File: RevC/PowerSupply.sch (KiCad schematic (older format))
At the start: 26 parts, among them Q21 DMG2301L, U22 TPS54202, U23 L7805, U24 MCP1754ST-3302E/CB, U25 NCP51460SN33T1G

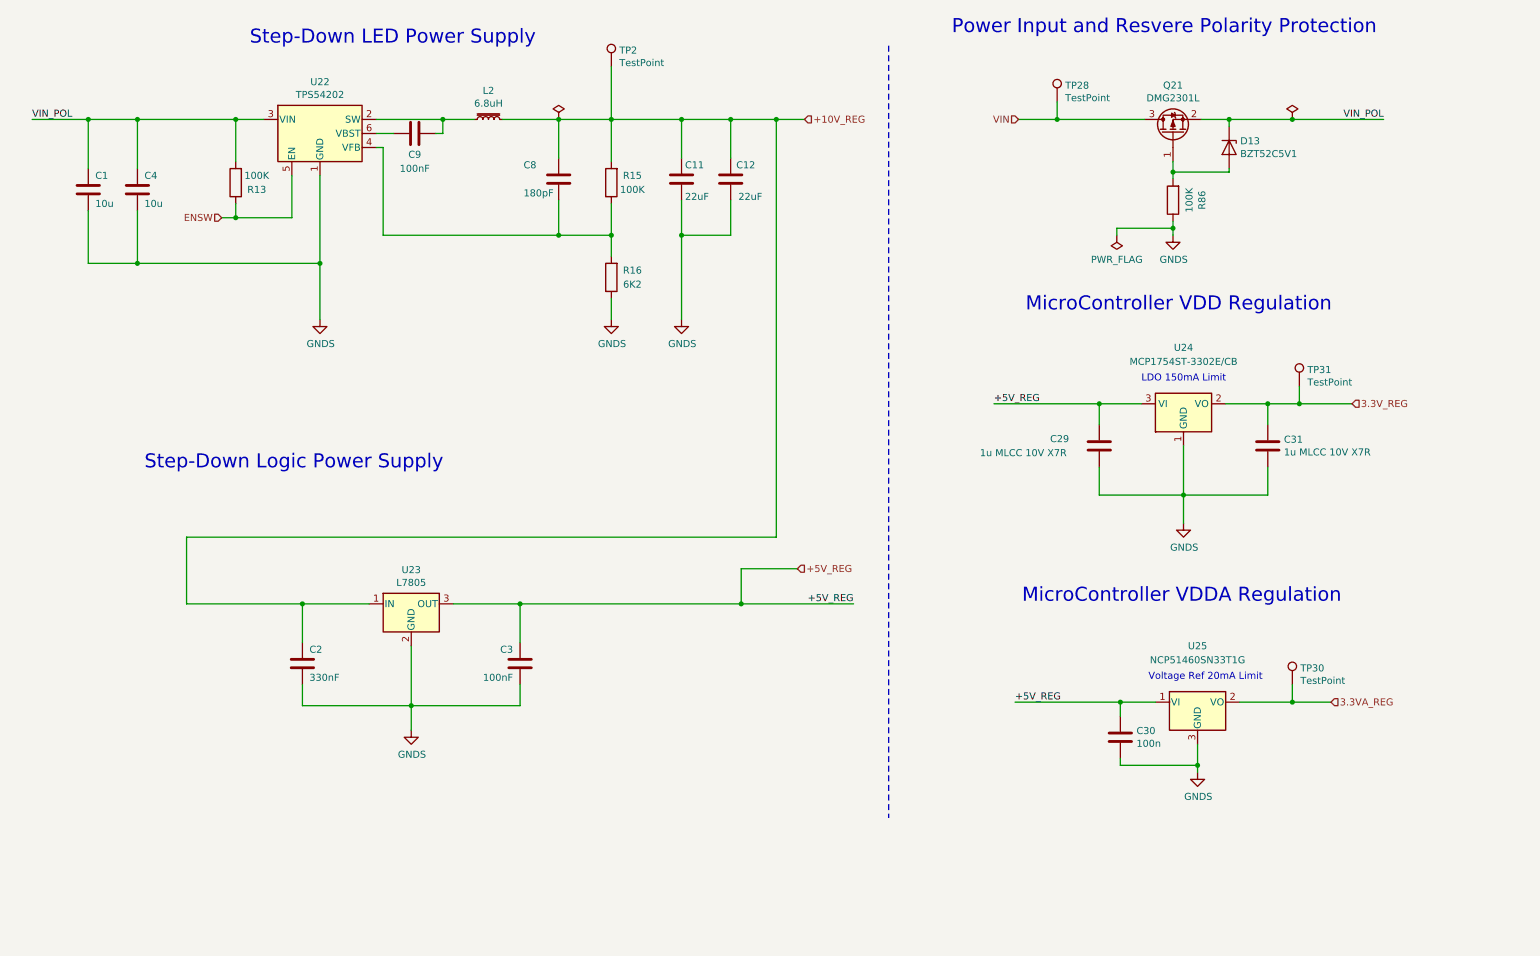
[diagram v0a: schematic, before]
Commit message: updates
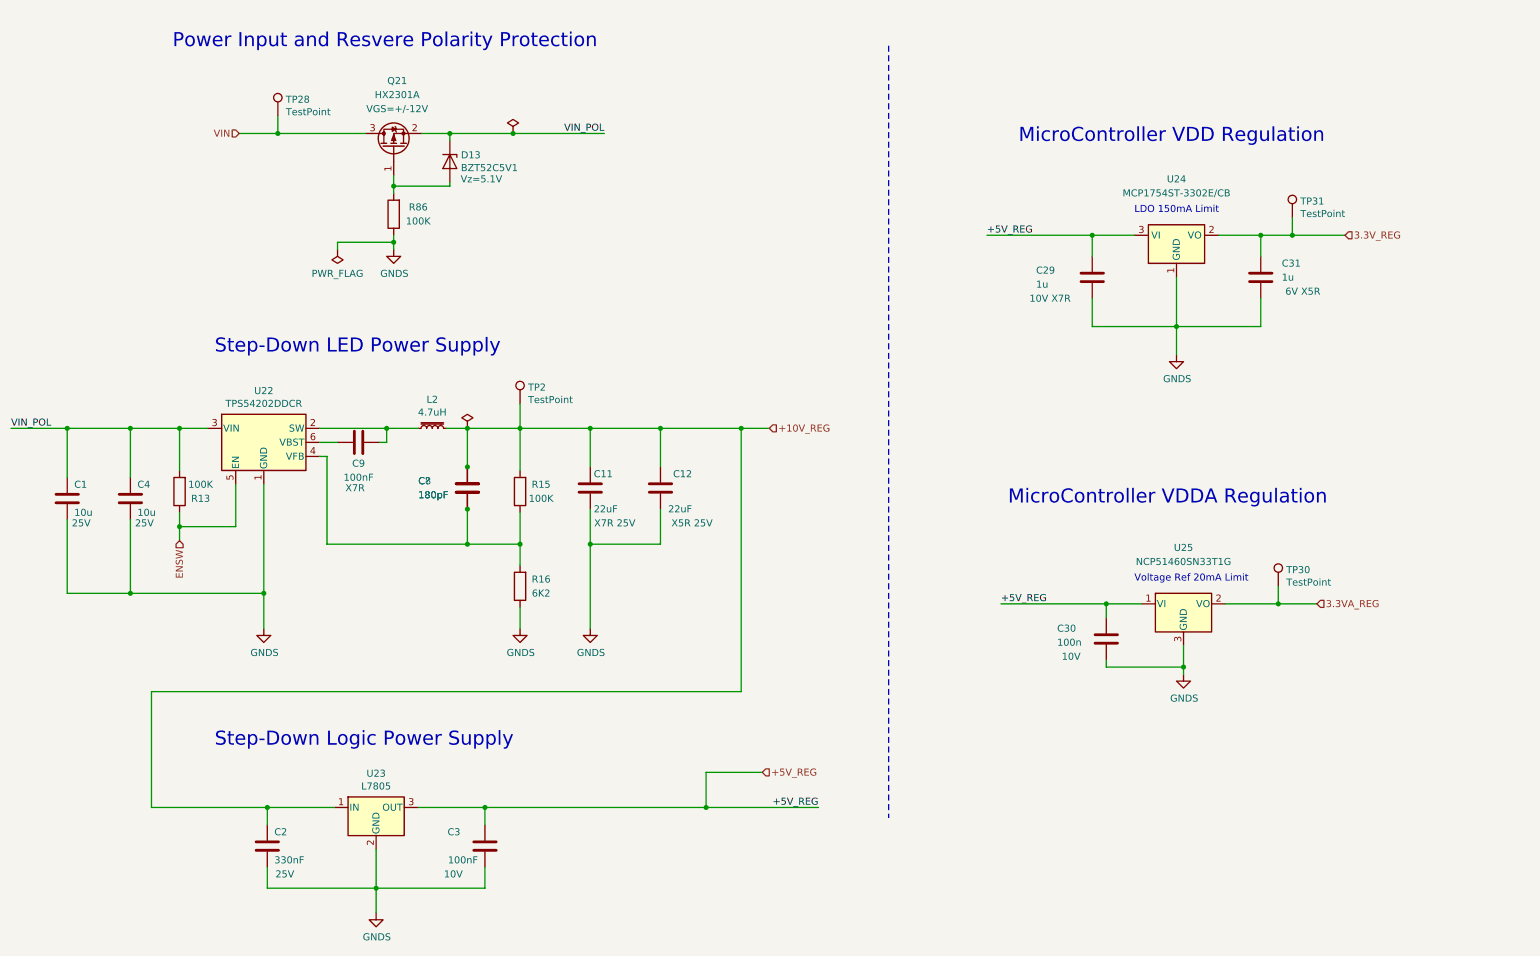
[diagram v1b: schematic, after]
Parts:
- added C?: 180pF, Resistor_SMD:R_0805_2012Metric_Pad1.15x1.40mm_HandSolder, symbol Device:C
- C1, C4: LcscNo (none) -> C14860; MouserNo 81-GRM21BC81C106KE5L -> (none)
- C11: LcscNo (none) -> C268007; MouserNo 810-C3216X5R1A476M -> (none); Type X5R, 2mΩ, 0.29A RMS, 4A -> X7R 25V
- C12: LcscNo (none) -> C268007; MouserNo 810-C3216X5R1A476M -> (none); Type X5R, 2mΩ, 0.29A RMS, 4A -> X5R 25V
- C2: LcscNo (none) -> C73142
- C29: value 1u MLCC 10V X7R -> 1u; LcscNo (none) -> C376927; MouserNo 80-C0805C105K3R -> (none); Type (none) -> 10V X7R
- C3: LcscNo (none) -> C94108
- C30: LcscNo (none) -> C94108; MouserNo 963-UMK212BJ104KG-T -> (none); Type (none) -> 10V
- C31: value 1u MLCC 10V X7R -> 1u; LcscNo (none) -> C376927; MouserNo 80-C0805C105K3R -> (none)
- C8: LcscNo (none) -> C152881; MouserNo 810-C3216X5R1A476M -> (none); Type (none) -> N/A
- C9: LcscNo (none) -> C94108; MouserNo 710-885012207098 -> (none); Type (none) -> X7R
- D13: LcscNo (none) -> C353516; MouserNo 771-BZT52-C5V1J -> (none); Type (none) -> Vz=5.1V
- L2: value 6.8uH -> 4.7uH; LcscNo (none) -> C266428; MouserNo 963-NRS8030T3R3MJGJ -> (none); Type (none) -> 3A
- Q21: value DMG2301L -> HX2301A; LcscNo (none) -> C296298; Type (none) -> VGS=+/-12V
- R13: LcscNo (none) -> C118844; MouserNo 71-CRCW080510K0FKEAC -> (none); Type (none) -> N/A
- R15: LcscNo (none) -> C118844; MouserNo 652-CR0805JW-563ELF -> (none); Type (none) -> N/A
- R16: Type (none) -> N/A
- R86: LcscNo (none) -> C118844; MouserNo 71-CRCW1206100KFKEAC -> (none); Type (none) -> N/A
- U22: value TPS54202 -> TPS54202DDCR; LcscNo (none) -> C191884; MouserNo 595-TPS54202DDCR -> (none)
- U23: LcscNo (none) -> C15077
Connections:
- net +10V_REG: now also C?.1
- net at C8.2, R15.1, R16.2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: now also C?.2
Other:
- moved on the sheet: C1, C11, C12, C2, C29, C3, C30, C31, C4, C8, C9, D13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
